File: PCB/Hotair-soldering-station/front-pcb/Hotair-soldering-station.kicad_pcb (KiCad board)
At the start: 2 copper layers, 54 parts, among them J1 fan_reg_pot, J2 main-board-conn, J3 hot_on, J4 solder_on, Q1 BC817, Q10 BC807, Q11 BC807, Q12 BC807, Q13 BC807, Q14 BC807, Q2 BC817, Q3 BC817, Q4 BC817, Q5 BC817, Q6 BC817, Q7 BC817, Q8 BC817, Q9 BC807, SW1 HOTAIR_UP, SW2 HOTAIR_DOWN, SW3 SIRON_UP, SW4 SIRON_DOWN, U1 74HC595D, U2 74HC595D, U3 My-Footprints:3-digit-7-segme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, U4 3-dig-7-seg-display-common-an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

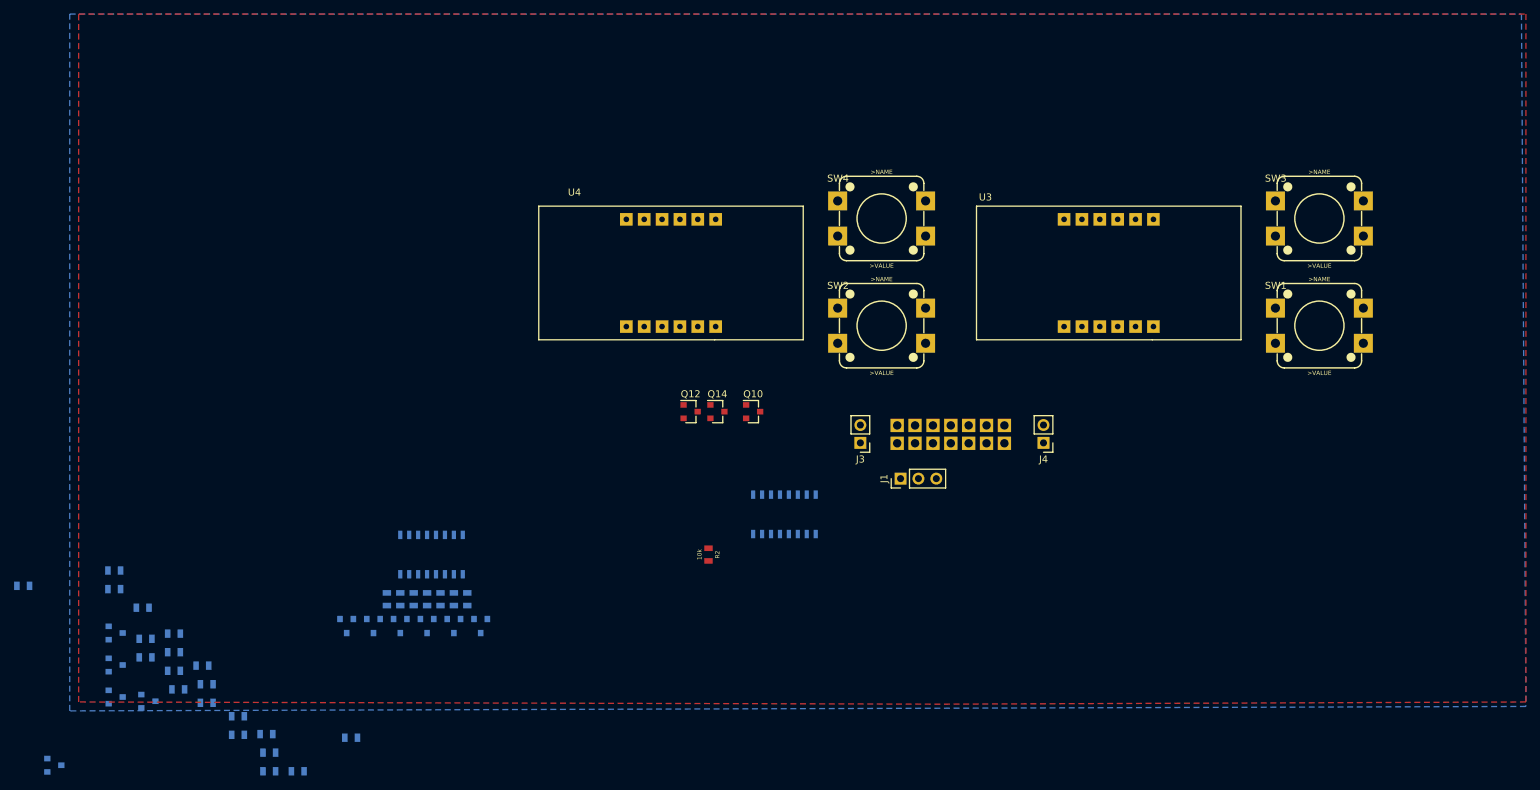
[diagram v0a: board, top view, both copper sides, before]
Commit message: routing progress
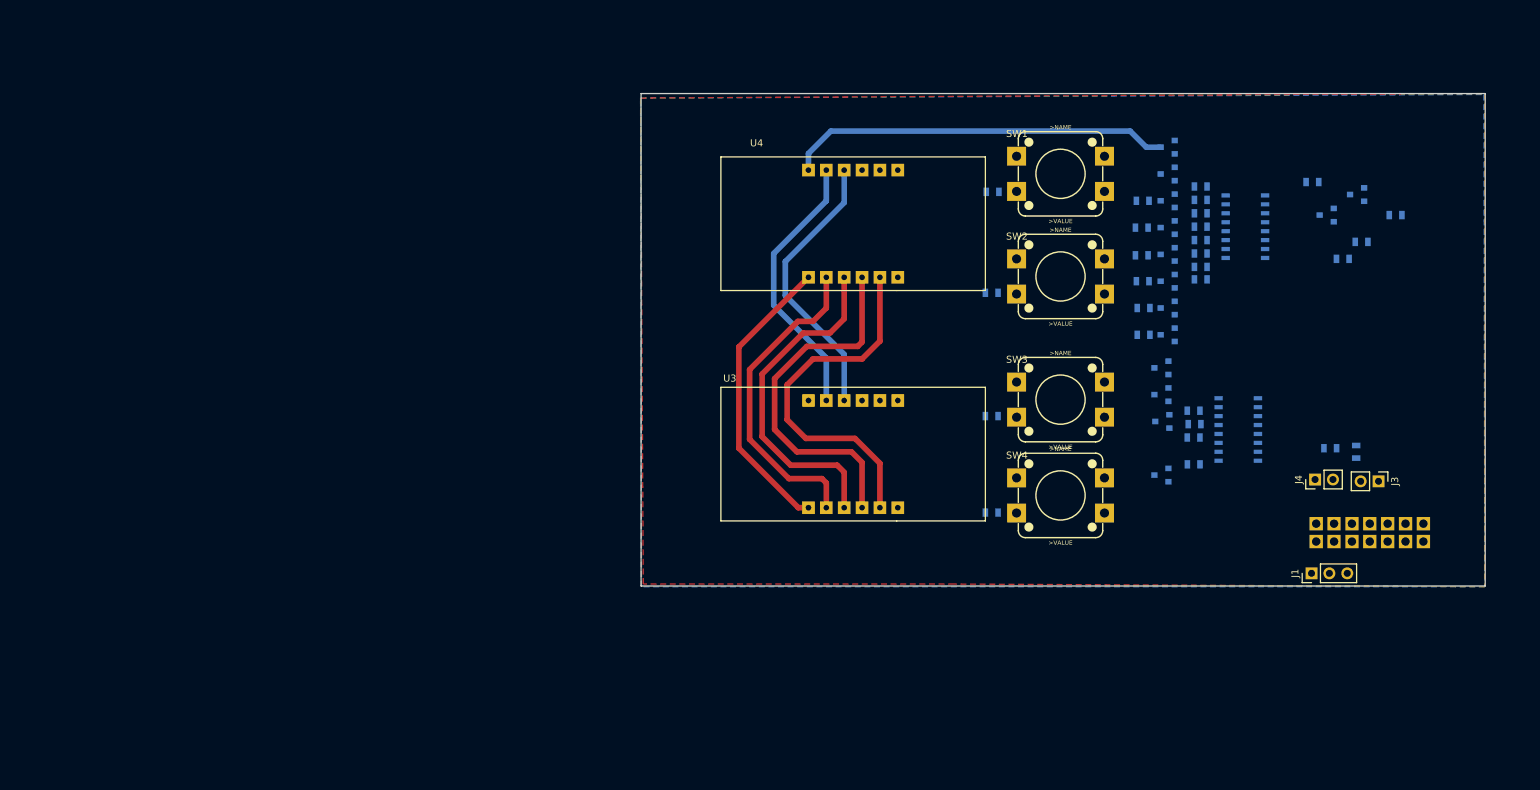
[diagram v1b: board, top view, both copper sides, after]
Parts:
- Q10, Q12, Q14, R2: moved to B.Cu
- moved Q7 186.3 mm to (200.8, 38.4), turned to 180 degrees
- moved Q8 185.3 mm to (196.5, 41.3), turned to 180 degrees
- moved R15 182.7 mm to (206.3, 41.3), turned to 180 degrees
- moved R16 171.0 mm to (198.8, 47.5), turned to 180 degrees
- moved R27 166.8 mm to (200.7, 74.9), turned to 90 degrees
- moved Q11 164.9 mm to (173.1, 70.6), turned to 180 degrees
- moved R28 163.2 mm to (197.0, 74.4)
- moved R22 161.9 mm to (178.6, 37.2)
- moved R20 159.5 mm to (178.6, 39.1)
- moved R17 155.4 mm to (177.7, 71.0)
- moved Q9 154.5 mm to (173.0, 63.0), turned to 180 degrees
- moved R13 153.2 mm to (170.2, 43.1), turned to 180 degrees
- moved R14 153.1 mm to (170.3, 39.2), turned to 180 degrees
- moved R11 151.5 mm to (170.3, 50.7), turned to 180 degrees
- moved R10 151.0 mm to (170.4, 54.5), turned to 180 degrees
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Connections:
- net Net-(R17-Pad2) renamed IRON_DIG2
- net Net-(R19-Pad2) renamed HOTAIR_DIG2
- R1 pad 1: Net-(R1-Pad1) -> SEG_DP
- R18 pad 2: Net-(R18-Pad2) -> IRON_DIG3
- R2 pad 1: Net-(R2-Pad1) -> SEG_G
- R20 pad 2: Net-(R20-Pad2) -> HOTAIR_DIG3
- R21 pad 2: Net-(R21-Pad2) -> IRON_DIG1
- R22 pad 2: Net-(R22-Pad2) -> HOTAIR_DIG1
- R3 pad 1: Net-(R3-Pad1) -> SEG_F
- R4 pad 1: Net-(R4-Pad1) -> SEG_E
- R5 pad 1: Net-(R5-Pad1) -> SEG_D
- R6 pad 1: Net-(R6-Pad1) -> SEG_C
- R7 pad 1: Net-(R7-Pad1) -> SEG_B
- R8 pad 1: Net-(R8-Pad1) -> SEG_A
- U1 pad 1: Net-(R2-Pad1) -> SEG_B
- U1 pad 15: Net-(R1-Pad1) -> SEG_A
- U1 pad 2: Net-(R3-Pad1) -> SEG_C
- U1 pad 3: Net-(R4-Pad1) -> SEG_D
- U1 pad 4: Net-(R5-Pad1) -> SEG_E
- U1 pad 5: Net-(R6-Pad1) -> SEG_F
- U1 pad 6: Net-(R7-Pad1) -> HOTAIR_DIG3
- U1 pad 7: Net-(R8-Pad1) -> HOTAIR_DIG1
- U2 pad 15: Net-(R20-Pad2) -> SEG_DP
- U2 pad 2: Net-(R22-Pad2) -> SEG_G
- U2 pad 3: Net-(R18-Pad2) -> IRON_DIG1
- U2 pad 5: Net-(R21-Pad2) -> IRON_DIG3
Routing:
- net Net-(Q12-Pad3): track 0.00 -> 54.7 mm
- net Net-(R10-Pad2): track 0.00 -> 51.9 mm
- net Net-(R14-Pad2): track 0.00 -> 51.8 mm
- net Net-(R9-Pad2): track 0.00 -> 48.5 mm
- net Net-(R13-Pad2): track 0.00 -> 45.8 mm
- net Net-(R12-Pad2): track 0.00 -> 41.8 mm
- net Net-(R11-Pad2): track 0.00 -> 39.7 mm
- net Net-(R16-Pad2): track 0.00 -> 38.9 mm
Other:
- board outline added: 120 x 70 mm
- net class Default: clearance 0.2 -> 0.5
- rule trace_clearance: 0.2 -> 0.5
